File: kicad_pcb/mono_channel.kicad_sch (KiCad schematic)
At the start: 133 parts, among them IC1 OPA1679, IC10 NE5532, IC2 NE5532, IC4 NE5532, J10 Conn_01x02, J12 Conn_01x02, J2 Conn_01x05, J4 Conn_01x02, J6 Conn_01x03, J8 Conn_01x05

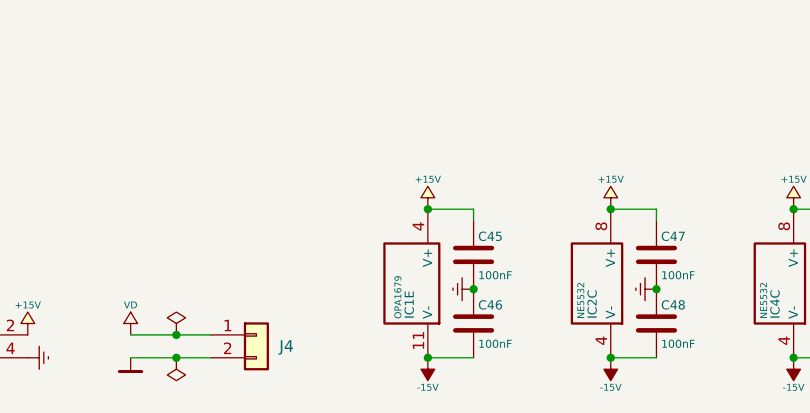
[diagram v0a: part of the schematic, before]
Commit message: fix
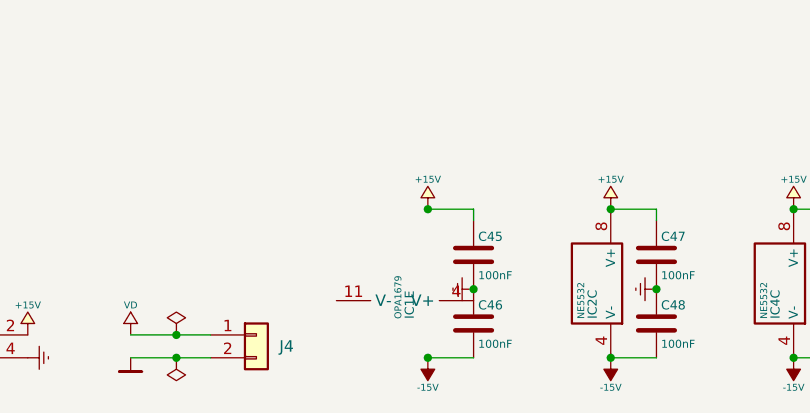
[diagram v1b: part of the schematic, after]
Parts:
- RELAY-2, RELAY-3, RELAY-4, RELAY-5: footprint 0_Switches:FTRB3GA45ZB10 -> 0_Switches:RELAY-2FORMC
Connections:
- net +15V: no longer IC1.4 (V+)
- net -15V: no longer IC1.11 (V-)
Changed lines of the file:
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@@
 			)
 		)
-		(property "Footprint" "0_Switches:FTRB3GA45ZB10"
+		(property "Footprint" "0_Switches:RELAY-2FORMC"
 			(at 368.554 193.548 0)
 			(hide yes)
@@
 			)
 		)
-		(property "Footprint" "0_Switches:FTRB3GA45ZB10"
+		(property "Footprint" "0_Switches:RELAY-2FORMC"
 			(at 128.016 164.338 0)
 			(hide yes)
@@
 			)
 		)
-		(property "Footprint" "0_Switches:FTRB3GA45ZB10"
+		(property "Footprint" "0_Switches:RELAY-2FORMC"
 			(at 148.844 164.338 0)
 			(hide yes)
@@
 			)
 		)
-		(property "Footprint" "0_Switches:FTRB3GA45ZB10"
+		(property "Footprint" "0_Switches:RELAY-2FORMC"
 			(at 239.014 145.288 0)
 			(hide yes)
